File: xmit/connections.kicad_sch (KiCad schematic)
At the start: 9 parts, among them J1 Conn_Coaxial, J2 Conn_01x02, J3 Conn_01x02, J4 Conn_01x02, J5 Conn_01x02

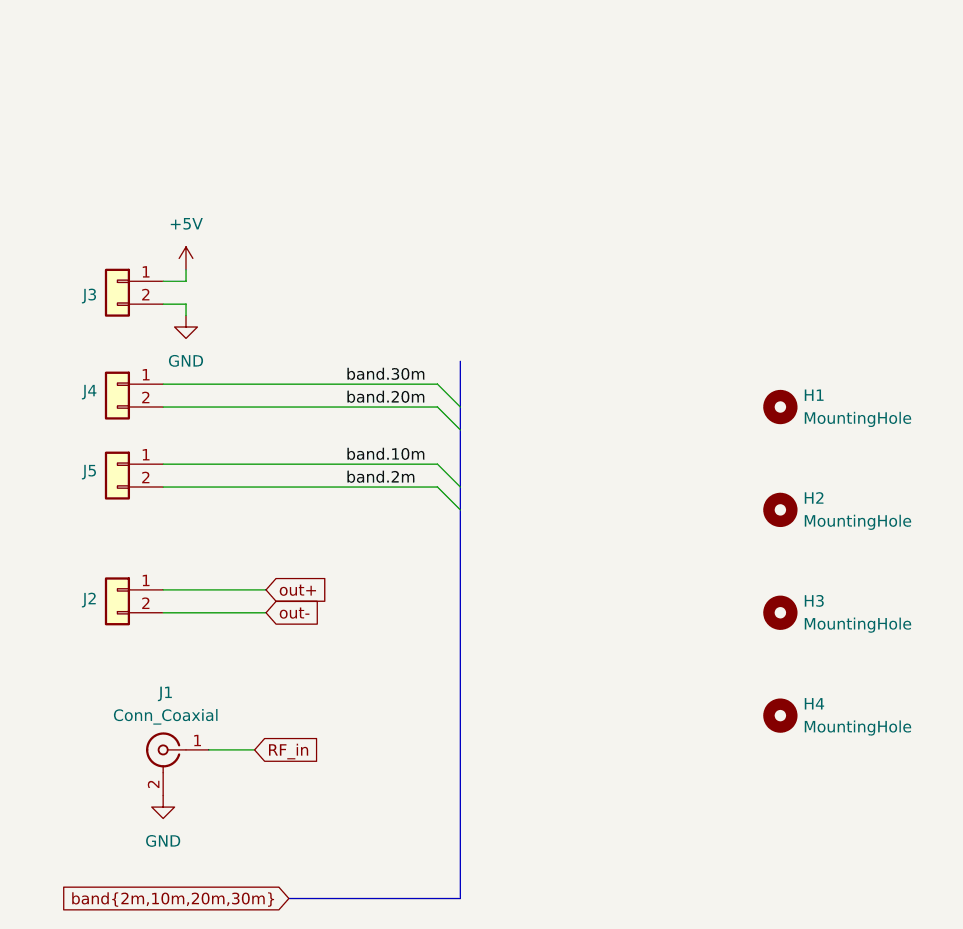
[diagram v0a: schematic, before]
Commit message: Another WIP on transmitter layout. Should be pretty close.
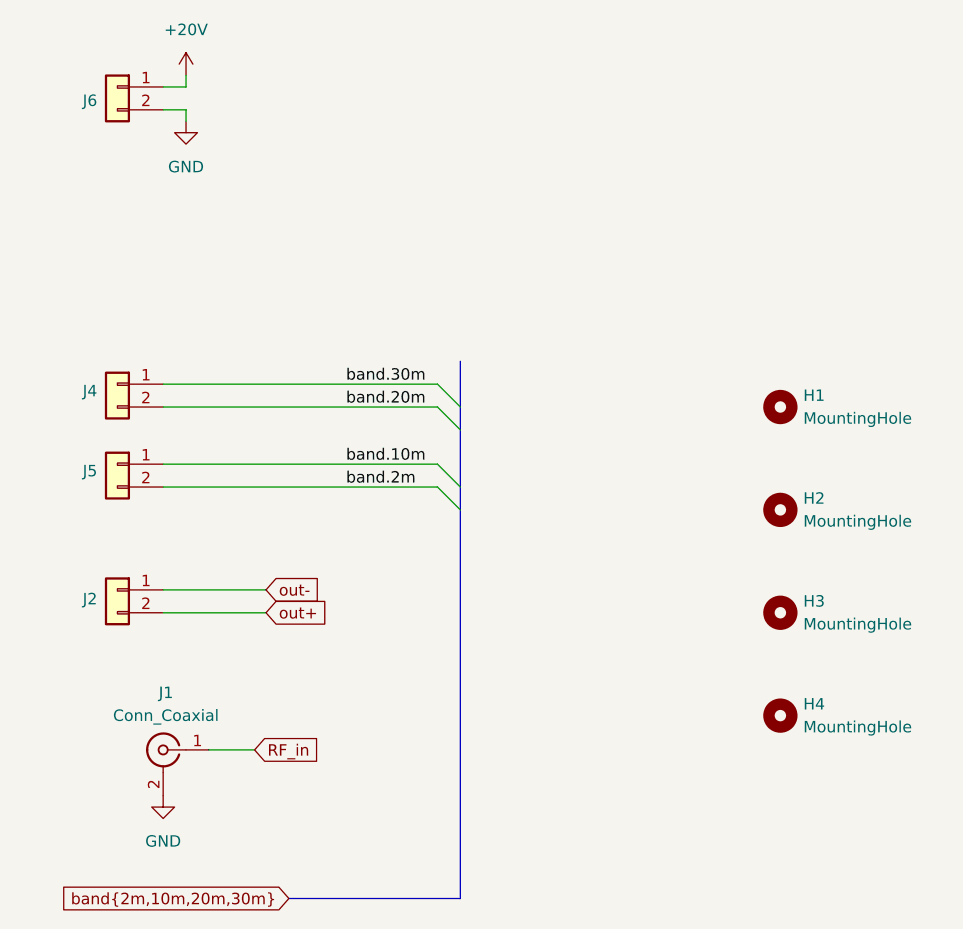
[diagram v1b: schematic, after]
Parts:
- removed J3: Conn_01x02, Connector_PinHeader_2.54mm:PinHeader_1x02_P2.54mm_Vertical, symbol Connector_Generic:Conn_01x02
- added J6: Conn_01x02, Connector:terminal_block_02, symbol Connector_Generic:Conn_01x02
- J1: footprint Connector_Coaxial:SMA_Molex_73251-1153_EdgeMount_Horizontal -> Connector_Coaxial:SMA_Samtec_SMA-J-P-H-ST-EM1_EdgeMount
- J2, J4, J5: footprint Connector_PinHeader_2.54mm:PinHeader_1x02_P2.54mm_Vertical -> Connector:terminal_block_02
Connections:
- net GND: now also J6.2 (Pin_2)
- net out+: now also J2.2 (Pin_2); no longer J2.1 (Pin_1)
- net out-: now also J2.1 (Pin_1); no longer J2.2 (Pin_2)
- new net +20V: J6.1 (Pin_1)
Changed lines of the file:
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@@
 	(wire
 		(pts
-			(xy 69.85 55.88) (xy 69.85 57.15)
+			(xy 69.85 34.29) (xy 69.85 35.56)
 		)
 		(stroke
@@
 	(wire
 		(pts
-			(xy 72.39 109.22) (xy 77.47 109.22)
+			(xy 69.85 35.56) (xy 67.31 35.56)
 		)
 		(stroke
@@
 	(wire
 		(pts
-			(xy 69.85 57.15) (xy 67.31 57.15)
+			(xy 72.39 109.22) (xy 77.47 109.22)
 		)
 		(stroke
@@
 	(wire
 		(pts
-			(xy 67.31 59.69) (xy 69.85 59.69)
+			(xy 67.31 38.1) (xy 69.85 38.1)
 		)
 		(stroke
@@
 	(wire
 		(pts
-			(xy 69.85 59.69) (xy 69.85 60.96)
+			(xy 69.85 38.1) (xy 69.85 39.37)
 		)
 		(stroke
@@
 		)
 	)
-	(global_label "out+"
+	(global_label "out-"
 		(shape input)
 		(at 78.74 91.44 0)
@@
 		)
 	)
-	(global_label "out-"
+	(global_label "out+"
 		(shape input)
 		(at 78.74 93.98 0)
@@
 				)
 				(justify left)
+			)
+		)
+	)
+	(symbol
+		(lib_id "Connector_Generic:Conn_01x02")
+		(at 62.23 35.56 0)
+		(mirror y)
+		(unit 1)
+		(body_style 1)
+		(exclude_from_sim no)
+		(in_bom yes)
+		(on_board yes)
+		(in_pos_files yes)
+		(dnp no)
+		(property "Reference" "J6"
+			(at 59.182 37.084 0)
+			(show_name no)
+			(do_not_autoplace no)
+			(effects
+				(font
+					(size 1.27 1.27)
+				)
+			)
+		)
+		(property "Value" "Conn_01x02"
+			(at 62.23 30.226 0)
+			(hide yes)
+			(show_name no)
+			(do_not_autoplace no)
+			(effects
+				(font
+					(size 1.27 1.27)
+				)
+			)
+		)
+		(property "Footprint" "Connector:terminal_block_02"
+			(at 62.23 35.56 0)
+			(hide yes)
+			(show_name no)
+			(do_not_autoplace no)
+			(effects
+				(font
+					(size 1.27 1.27)
+				)
+			)
+		)
+		(property "Datasheet" ""
+			(at 62.23 35.56 0)
+			(hide yes)
+			(show_name no)
+			(do_not_autoplace no)
+			(effects
+				(font
+					(size 1.27 1.27)
+				)
+			)
+		)
+		(property "Description" "Generic connector, single row, 01x02, script generated (kicad-library-utils/schlib/autogen/connector/)"
+			(at 62.23 35.56 0)
+			(hide yes)
+			(show_name no)
+			(do_not_autoplace no)
+			(effects
+				(font
+					(size 1.27 1.27)
+				)
+			)
+		)
+		(pin "2"
+		)
+		(pin "1"
+		)
+		(instances
+			(project "xmit"
+				(path "/938afe95-c1c4-4cca-88b7-71a9df9e4417/504c6b8f-78e0-414e-b95c-1cb18df8f301"
+					(reference "J6")
+					(unit 1)
+				)
 			)
 		)
@@
 	)
 	(symbol
+		(lib_id "power:+5V")
+		(at 69.85 34.29 0)
+		(unit 1)
+		(body_style 1)
+		(exclude_from_sim no)
+		(in_bom yes)
+		(on_board yes)
+		(in_pos_files yes)
+		(dnp no)
+		(fields_autoplaced yes)
+		(property "Reference" "#PWR036"
+			(at 69.85 38.1 0)
+			(hide yes)
+			(show_name no)
+			(do_not_autoplace no)
+			(effects
+				(font
+					(size 1.27 1.27)
+				)
+			)
+		)
+		(property "Value" "+20V"
+			(at 69.85 29.21 0)
+			(show_name no)
+			(do_not_autoplace no)
+			(effects
+				(font
+					(size 1.27 1.27)
+				)
+			)
+		)
+		(property "Footprint" ""
+			(at 69.85 34.29 0)
+			(hide yes)
+			(show_name no)
+			(do_not_autoplace no)
+			(effects
+				(font
+					(size 1.27 1.27)
+				)
+			)
+		)
+		(property "Datasheet" ""
+			(at 69.85 34.29 0)
+			(hide yes)
+			(show_name no)
+			(do_not_autoplace no)
+			(effects
+				(font
+					(size 1.27 1.27)
+				)
+			)
+		)
+		(property "Description" "Power symbol creates a global label with name \"+5V\""
+			(at 69.85 34.29 0)
+			(hide yes)
+			(show_name no)
+			(do_not_autoplace no)
+			(effects
+				(font
+					(size 1.27 1.27)
+				)
+			)
+		)
+		(pin "1"
+		)
+		(instances
+			(project "xmit"
+				(path "/938afe95-c1c4-4cca-88b7-71a9df9e4417/504c6b8f-78e0-414e-b95c-1cb18df8f301"
+					(reference "#PWR036")
+					(unit 1)
+				)
+			)
+		)
+	)
+	(symbol
 		(lib_id "Mechanical:MountingHole")
 		(at 135.89 105.41 0)
@@
 	(symbol
 		(lib_id "power:GND")
-		(at 69.85 60.96 0)
+		(at 69.85 39.37 0)
 		(mirror y)
 		(unit 1)
@@
 		(in_pos_files yes)
 		(dnp no)
-		(property "Reference" "#PWR028"
-			(at 69.85 67.31 0)
+		(property "Reference" "#PWR038"
+			(at 69.85 45.72 0)
 			(hide yes)
 			(show_name no)
@@
 		)
 		(property "Value" "GND"
-			(at 69.85 66.04 0)
+			(at 69.85 44.45 0)
 			(show_name no)
 			(do_not_autoplace no)
@@
 		)
 		(property "Footprint" ""
-			(at 69.85 60.96 0)
+			(at 69.85 39.37 0)
 			(hide yes)
 			(show_name no)
@@
 		)
 		(property "Datasheet" ""
-			(at 69.85 60.96 0)
+			(at 69.85 39.37 0)
 			(hide yes)
 			(show_name no)
@@
 		)
 		(property "Description" "Power symbol creates a global label with name \"GND\" , ground"
-			(at 69.85 60.96 0)
+			(at 69.85 39.37 0)
 			(hide yes)
 			(show_name no)
@@
 			(project "xmit"
 				(path "/938afe95-c1c4-4cca-88b7-71a9df9e4417/504c6b8f-78e0-414e-b95c-1cb18df8f301"
-					(reference "#PWR028")
+					(reference "#PWR038")
 					(unit 1)
 				)
@@
 			)
 		)
-		(property "Footprint" "Connector_Coaxial:SMA_Molex_73251-1153_EdgeMount_Horizontal"
+		(property "Footprint" "Connector_Coaxial:SMA_Samtec_SMA-J-P-H-ST-EM1_EdgeMount"
 			(at 67.31 109.22 0)
 			(hide yes)
@@
 			)
 		)
-		(property "Footprint" "Connector_PinHeader_2.54mm:PinHeader_1x02_P2.54mm_Vertical"
+		(property "Footprint" "Connector:terminal_block_02"
 			(at 62.23 77.47 0)
 			(hide yes)
@@
 			)
 		)
-		(property "Footprint" "Connector_PinHeader_2.54mm:PinHeader_1x02_P2.54mm_Vertical"
+		(property "Footprint" "Connector:terminal_block_02"
 			(at 62.23 91.44 0)
 			(hide yes)
@@
 				(path "/938afe95-c1c4-4cca-88b7-71a9df9e4417/504c6b8f-78e0-414e-b95c-1cb18df8f301"
 					(reference "J2")
-					(unit 1)
-				)
-			)
-		)
-	)
-	(symbol
-		(lib_id "power:+5V")
-		(at 69.85 55.88 0)
-		(unit 1)
-		(body_style 1)
-		(exclude_from_sim no)
-		(in_bom yes)
-		(on_board yes)
-		(in_pos_files yes)
-		(dnp no)
-		(fields_autoplaced yes)
-		(property "Reference" "#PWR029"
-			(at 69.85 59.69 0)
-			(hide yes)
-			(show_name no)
-			(do_not_autoplace no)
-			(effects
-				(font
-					(size 1.27 1.27)
-				)
-			)
-		)
-		(property "Value" "+5V"
-			(at 69.85 50.8 0)
-			(show_name no)
-			(do_not_autoplace no)
-			(effects
-				(font
-					(size 1.27 1.27)
-				)
-			)
-		)
-		(property "Footprint" ""
-			(at 69.85 55.88 0)
-			(hide yes)
-			(show_name no)
-			(do_not_autoplace no)
-			(effects
-				(font
-					(size 1.27 1.27)
-				)
-			)
-		)
-		(property "Datasheet" ""
-			(at 69.85 55.88 0)
-			(hide yes)
-			(show_name no)
-			(do_not_autoplace no)
-			(effects
-				(font
-					(size 1.27 1.27)
-				)
-			)
-		)
-		(property "Description" "Power symbol creates a global label with name \"+5V\""
-			(at 69.85 55.88 0)
-			(hide yes)
-			(show_name no)
-			(do_not_autoplace no)
-			(effects
-				(font
-					(size 1.27 1.27)
-				)
-			)
-		)
-		(pin "1"
-		)
-		(instances
-			(project "xmit"
-				(path "/938afe95-c1c4-4cca-88b7-71a9df9e4417/504c6b8f-78e0-414e-b95c-1cb18df8f301"
-					(reference "#PWR029")
 					(unit 1)
 				)
@@
 			)
 		)
-		(property "Footprint" "Connector_PinHeader_2.54mm:PinHeader_1x02_P2.54mm_Vertical"
+		(property "Footprint" "Connector:terminal_block_02"
 			(at 62.23 68.58 0)
 			(hide yes)
@@
 					(unit 1)
 				)
-			)
-		)
-	)
-	(symbol
-		(lib_id "Connector_Generic:Conn_01x02")
-		(at 62.23 57.15 0)
-		(mirror y)
-		(unit 1)
-		(body_style 1)
-		(exclude_from_sim no)
-		(in_bom yes)
-		(on_board yes)
-		(in_pos_files yes)
-		(dnp no)
-		(property "Reference" "J3"
-			(at 59.182 58.674 0)
-			(show_name no)
-			(do_not_autoplace no)
-			(effects
-				(font
-					(size 1.27 1.27)
-				)
-			)
-		)
-		(property "Value" "Conn_01x02"
-			(at 62.23 51.816 0)
-			(hide yes)
-			(show_name no)
-			(do_not_autoplace no)
-			(effects
-				(font
-					(size 1.27 1.27)
-				)
-			)
-		)
-		(property "Footprint" "Connector_PinHeader_2.54mm:PinHeader_1x02_P2.54mm_Vertical"
-			(at 62.23 57.15 0)
-			(hide yes)
-			(show_name no)
-			(do_not_autoplace no)
-			(effects
-				(font
-					(size 1.27 1.27)
-				)
-			)
-		)
-		(property "Datasheet" ""
-			(at 62.23 57.15 0)
-			(hide yes)
-			(show_name no)
-			(do_not_autoplace no)
-			(effects
-				(font
-					(size 1.27 1.27)
-				)
-			)
-		)
-		(property "Description" "Generic connector, single row, 01x02, script generated (kicad-library-utils/schlib/autogen/connector/)"
-			(at 62.23 57.15 0)
-			(hide yes)
-			(show_name no)
-			(do_not_autoplace no)
-			(effects
-				(font
-					(size 1.27 1.27)
-				)
-			)
-		)
-		(pin "2"
-		)
-		(pin "1"
-		)
-		(instances
-			(project "xmit"
-				(path "/938afe95-c1c4-4cca-88b7-71a9df9e4417/504c6b8f-78e0-414e-b95c-1cb18df8f301"
-					(reference "J3")
-					(unit 1)
-				)
